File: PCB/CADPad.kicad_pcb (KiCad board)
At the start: 2 copper layers, 33 parts, among them SW1 SW_Push, SW10 RotaryEncoder_Switch, SW2 SW_Push, SW3 SW_Push, SW4 SW_Push, SW5 SW_Push, SW6 SW_Push, SW7 SW_Push, SW8 SW_Push, SW9 SW_Push, U1 XIAO-RP2040-DIP

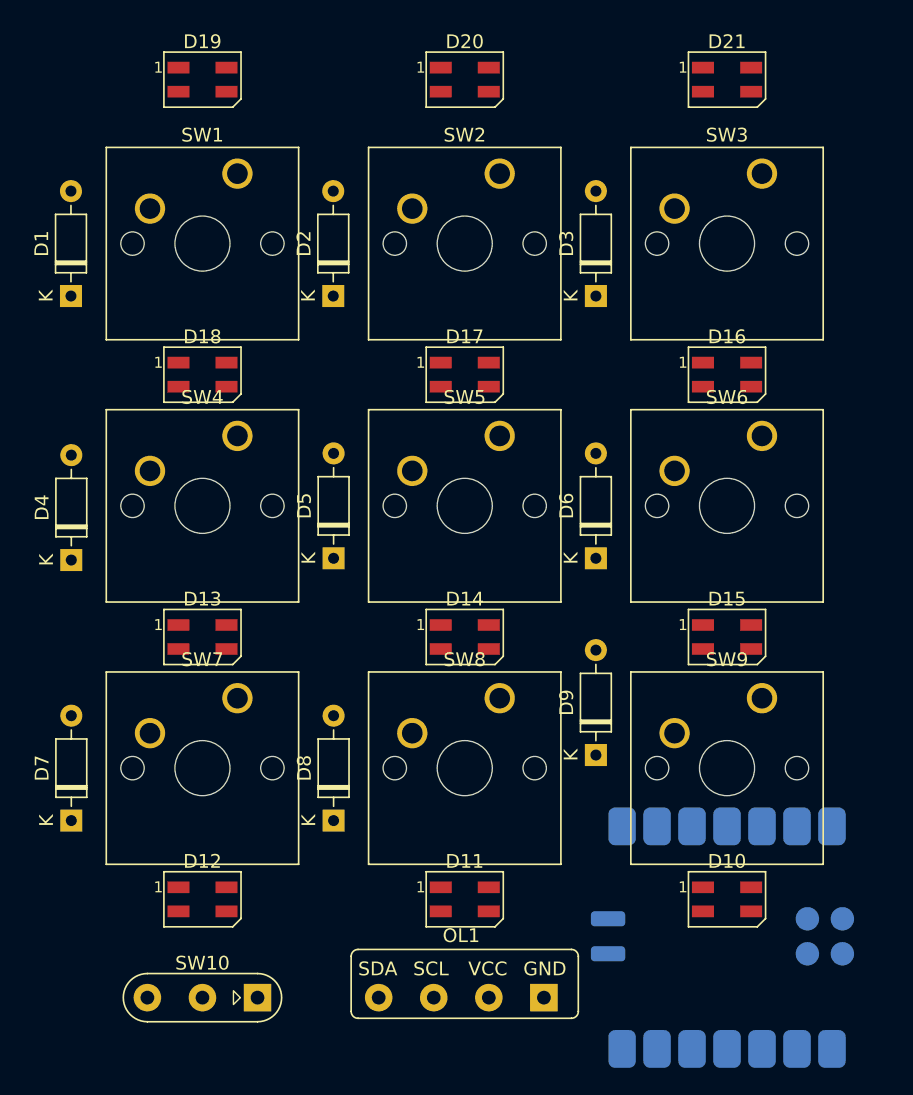
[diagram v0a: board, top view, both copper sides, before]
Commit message: traced almost everything
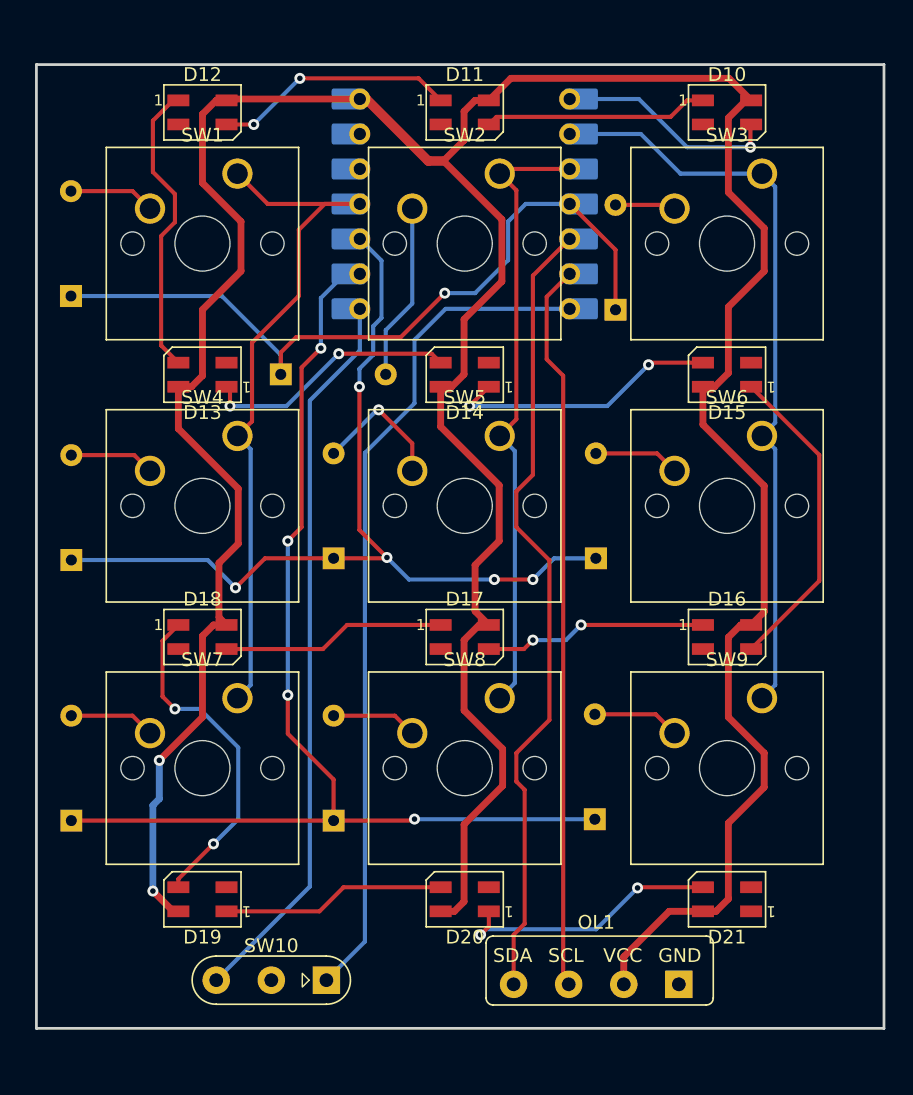
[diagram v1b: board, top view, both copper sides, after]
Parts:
- D1, D2, D3, D4, D5, D6, D7, D8, D9: moved to B.Cu
- U1: footprint OPL:XIAO-RP2040-SMD -> OPL:XIAO-RP2040-DIP
- moved D19 59.5 mm to (124.7, 125.7), turned to 180 degrees
- moved D20 59.5 mm to (143.8, 125.7), turned to 180 degrees
- moved D21 59.5 mm to (162.8, 125.7), turned to 180 degrees
- moved D10 57.2 mm to (162.8, 68.6)
- moved D11 57.2 mm to (143.8, 68.6)
- moved D12 57.2 mm to (124.7, 68.6)
- moved U1 56.7 mm to (143.8, 75.2), turned to 180 degrees
- moved D13 19.1 mm to (124.7, 87.6), turned to 180 degrees
- moved D14 19.1 mm to (143.8, 87.6), turned to 180 degrees
- moved D15 19.1 mm to (162.8, 87.6), turned to 180 degrees
- moved D16 19.1 mm to (162.8, 106.7)
- moved D17 19.1 mm to (143.8, 106.7)
- moved D18 19.1 mm to (124.7, 106.7)
- moved OL1 9.85 mm to (147.3, 131.9)
- moved D2 6.85 mm to (130.4, 87.6), turned to 0 degrees
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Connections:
- U1 pad 1: ROW 0 -> LED
- U1 pad 10: COL 0 -> ROW 1
- U1 pad 11: LED -> COL 0
- U1 pad 2: ROW 1 -> COL 2
- U1 pad 3: ROW 2 -> COL 1
- U1 pad 4: EC11 A -> ROW 0
- U1 pad 7: EC11 B -> EC11 A
- U1 pad 8: COL 2 -> EC11 B
- U1 pad 9: COL 1 -> ROW 2
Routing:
- net +5V: track 0.00 -> 259.8 mm, vias 0 -> 2
- net ROW 2: track 0.00 -> 82.0 mm, vias 0 -> 4
- net ROW 1: track 0.00 -> 66.4 mm, vias 0 -> 5
- net EC11 A: track 0.00 -> 61.4 mm
- net SDA: track 0.00 -> 58.3 mm
- net ROW 0: track 0.00 -> 56.2 mm, vias 0 -> 1
- net COL 2: track 0.00 -> 54.9 mm
- net EC11 B: track 0.00 -> 53.1 mm
- net SCL: track 0.00 -> 53.0 mm
- net COL 0: track 0.00 -> 51.7 mm
- net COL 1: track 0.00 -> 45.2 mm
- net Net-(D18-DOUT): track 0.00 -> 24.7 mm, vias 0 -> 2
- net Net-(D15-DOUT): track 0.00 -> 23.2 mm
- net Net-(D12-DOUT): track 0.00 -> 21.6 mm
- net Net-(D14-DOUT): track 0.00 -> 20.2 mm, vias 0 -> 2
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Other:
- board outline added: 61.6 x 70 mm
- board text removed: "XIAO HERE"
